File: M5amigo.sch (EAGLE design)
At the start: 2 parts, among them CN1 CON_PINHD-2X15, CN2 CON_PINHD-2X15

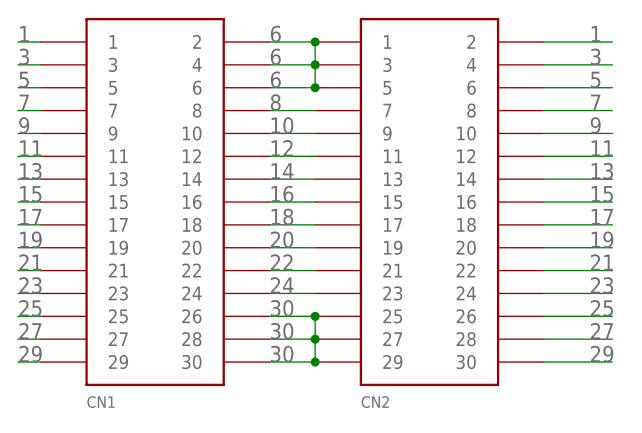
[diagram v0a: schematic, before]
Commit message: better Pinout understanding !
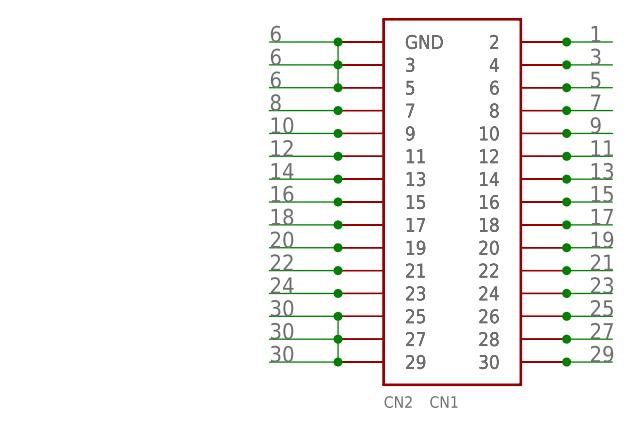
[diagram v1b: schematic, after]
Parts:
- CN1: value CON_PINHD-2X15 -> CON_PINHD-2X15_BOTTOM; device akita:CON_PINHD-2X15 -> akita:CON_PINHD-2X15_BOTTOM
- CN2: value CON_PINHD-2X15 -> CON_PINHD-2X15_TOP; device akita:CON_PINHD-2X15 -> akita:CON_PINHD-2X15_TOP
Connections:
- net 1: now also CN1.2; no longer CN1.1
- net 10: now also CN1.9; no longer CN1.10
- net 11: now also CN1.12; no longer CN1.11
- net 12: now also CN1.11; no longer CN1.12
- net 13: now also CN1.14; no longer CN1.13
- net 14: now also CN1.13; no longer CN1.14
- net 15: now also CN1.16; no longer CN1.15
- net 16: now also CN1.15; no longer CN1.16
- net 17: now also CN1.18; no longer CN1.17
- net 18: now also CN1.17; no longer CN1.18
- net 19: now also CN1.20; no longer CN1.19
- net 20: now also CN1.19; no longer CN1.20
- net 21: now also CN1.22; no longer CN1.21
- net 22: now also CN1.21; no longer CN1.22
- net 23: now also CN1.24; no longer CN1.23
- net 24: now also CN1.23; no longer CN1.24
- net 25: now also CN1.26; no longer CN1.25
- net 27: now also CN1.28; no longer CN1.27
- net 29: now also CN1.30; no longer CN1.29
- net 3: now also CN1.4; no longer CN1.3
- net 30: now also CN1.25, CN1.27, CN1.29; no longer CN1.26, CN1.28, CN1.30
- net 5: now also CN1.6; no longer CN1.5
- net 6: now also CN1.3, CN1.5, CN1.GND, CN2.GND; no longer CN1.2, CN1.4, CN1.6, CN2.1
- net 7: now also CN1.8; no longer CN1.7
- net 8: now also CN1.7; no longer CN1.8
- net 9: now also CN1.10; no longer CN1.9
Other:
- moved on the sheet: CN1, CN2
